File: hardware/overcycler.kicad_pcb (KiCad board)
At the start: 2 copper layers, 99.1 x 104.1 mm, 42 parts, among them P1 LPC_P1, P10 VCA_CMD_PWR, P11 AC_IN, P12 FOOT_IN, P13 MIDI_IN, P2 LPC_P2, P3 FT232, P4 CARD0_CMD_PWR, P5 SDCARD, P6 CARD1_CMD_PWR, P7 SCREEN, P8 CARD2_CMD_PWR, P9 TEN_POTS, SW1 RESET, U1 4053, U2 4053, U3 MCP4921-E/P, U4 LM1084IT-5.0/NOPB, U5 LM2990-5.0/NOPB, U6 LM1084IT-3.3/NOPB

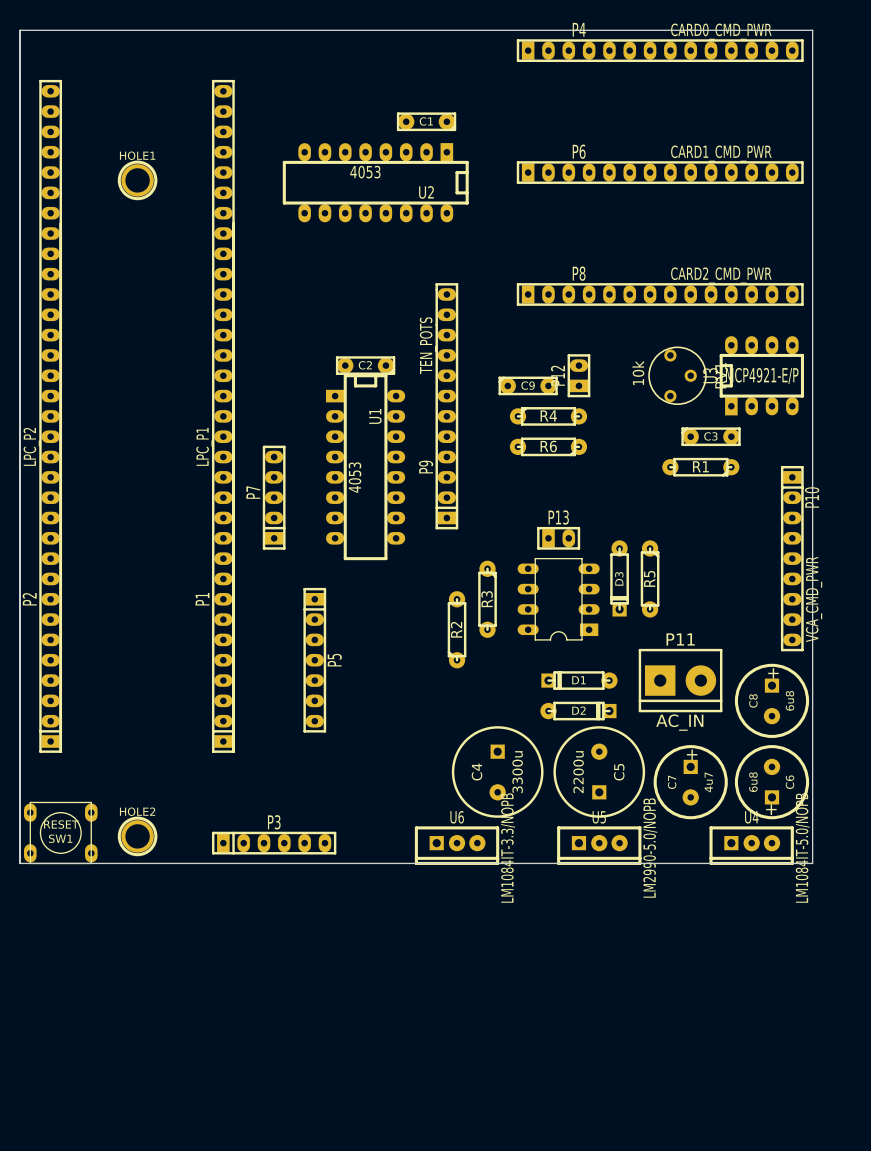
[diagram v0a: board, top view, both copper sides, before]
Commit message: mainboard almost ok
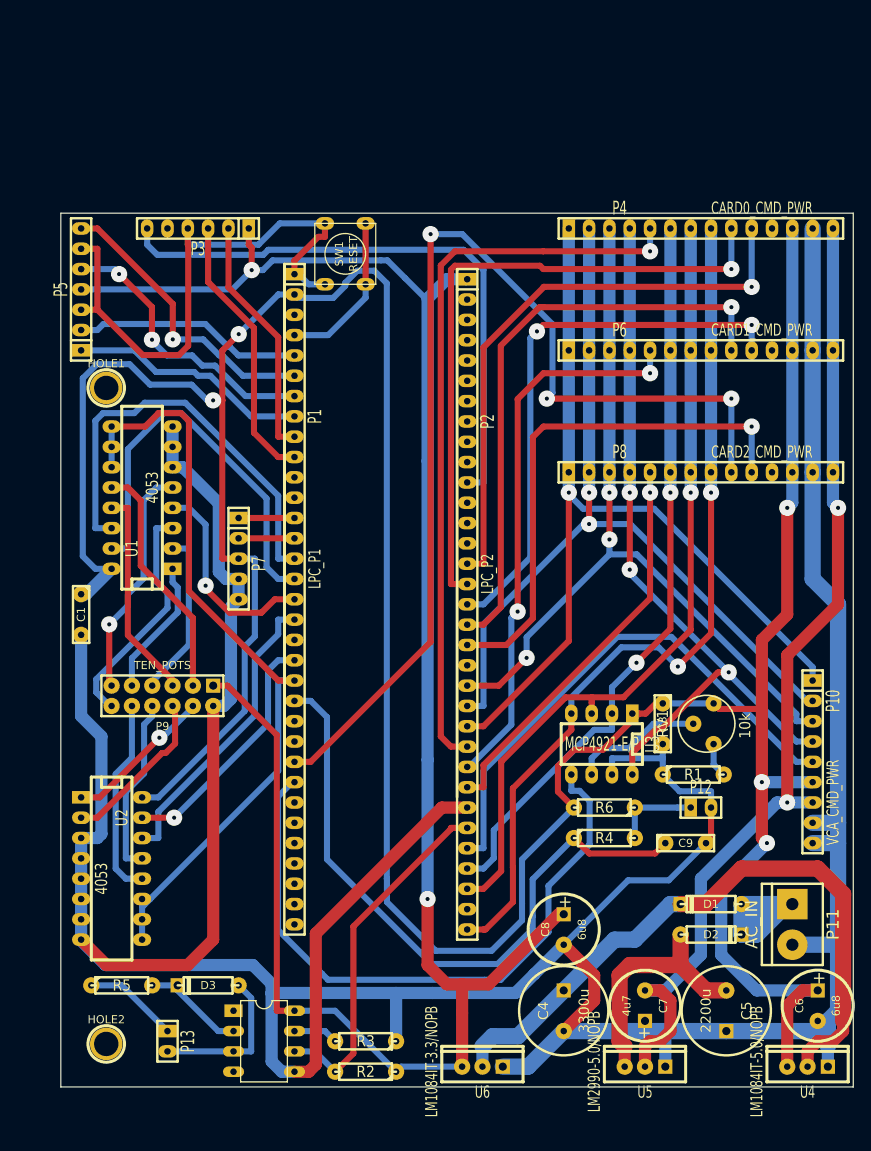
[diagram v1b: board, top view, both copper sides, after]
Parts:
- removed C2: 100n, C2
- P9: footprint SIL-12 -> pin_array_6x2
- moved U2 91.9 mm to (31.8, 120.0), turned to 270 degrees
- moved R5 83.3 mm to (33.0, 134.6), turned to 0 degrees
- moved SW1 80.7 mm to (61.0, 43.2), turned to 90 degrees
- moved P13 79.6 mm to (38.7, 141.6), turned to 270 degrees
- moved P3 77.4 mm to (42.5, 40.0), turned to 180 degrees
- moved C1 75.2 mm to (27.9, 88.3), turned to 270 degrees
- moved D3 72.3 mm to (43.8, 134.6), turned to 180 degrees
- moved OC1 66.4 mm to (50.8, 141.6), turned to 270 degrees
- moved C9 60.4 mm to (103.5, 116.8)
- moved R3 57.3 mm to (63.5, 141.6), turned to 180 degrees
- moved R2 56.4 mm to (63.5, 145.4), turned to 180 degrees
- moved P12 56.1 mm to (105.4, 112.4), turned to 0 degrees
- moved P5 54.8 mm to (27.9, 47.6), turned to 90 degrees
- moved R4 53.2 mm to (93.3, 116.2)
- moved P2 52.4 mm to (76.2, 78.1), turned to 270 degrees
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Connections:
- P10 pad 7: GND -> -5V
- P10 pad 9: -5V -> GND
- P2 pad 27: (no net) -> GND
- P9 pad 1: GND -> +3.3V
- P9 pad 10: N-0000010 (its old number) -> N-0000027
- P9 pad 11: N-0000011 (its old number) -> N-0000025
- P9 pad 12: N-000002 (its old number) -> N-0000026
- P9 pad 2: +3.3V -> GND
- P9 pad 4: N-000005 -> N-0000034
- P9 pad 5: N-000006 (its old number) -> N-0000022
- P9 pad 6: N-000007 -> N-000005
- P9 pad 7: N-000003 (its old number) -> N-0000023
- P9 pad 8: N-000008 -> N-0000028
- P9 pad 9: N-000009 (its old number) -> N-0000020
- U1 pad 1: N-000007 -> N-0000020
- U1 pad 13: N-000005 -> N-0000022
- U1 pad 2: N-000006 (its old number) -> N-0000023
- U1 pad 3: N-000008 -> N-0000026
- U1 pad 5: N-000003 (its old number) -> N-0000025
- U2 pad 1: N-000002 (its old number) -> N-0000034
- U2 pad 12: N-000009 (its old number) -> N-0000027
- U2 pad 13: N-0000010 (its old number) -> N-0000028
- U2 pad 2: N-0000011 (its old number) -> N-000005
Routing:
- net GND: track 0.00 -> 592.9 mm
- net +5V: track 0.00 -> 423.0 mm, vias 0 -> 5
- net +3.3V: track 0.00 -> 245.3 mm, vias 0 -> 2
- net N-0000045: track 0.00 -> 136.4 mm, vias 0 -> 3
- net -5V: track 0.00 -> 124.9 mm, vias 0 -> 2
- net N-0000040: track 0.00 -> 110.0 mm, vias 0 -> 1
- net N-000003: track 0.00 -> 109.1 mm, vias 0 -> 2
- net N-000002: track 0.00 -> 104.7 mm, vias 0 -> 2
- net N-000004: track 0.00 -> 101.6 mm, vias 0 -> 1
- net N-000001: track 0.00 -> 101.4 mm, vias 0 -> 3
- net N-0000024: track 0.00 -> 97.5 mm
- net /UNR+: track 0.00 -> 95.7 mm
- net N-0000041: track 0.00 -> 93.7 mm, vias 0 -> 3
- net N-000006: track 0.00 -> 93.0 mm, vias 0 -> 2
- net N-0000035: track 0.00 -> 92.5 mm, vias 0 -> 1
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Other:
- board size 99.1 x 104.1 mm -> 99.1 x 109.2 mm
- net class ac removed
- net class pwr removed
